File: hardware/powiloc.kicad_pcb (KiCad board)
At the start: 2 copper layers, 55.9 x 92.7 mm, 46 parts, among them J1 SW_PWR_BAT, J2 MCU_ISP, J3 SW_ISP_MCU, J4 neo_gps_conn, J5 oled_conn, J6 periph_conn_1, J7 BATT, J8 radio_ant_conn**, J9 MCU_TX, Q1 IRF740, Q2 IRF740, SW1 SW_TRIG, SW2 SW_MAIN_RST, SW3 SW_LED_PWR, SW4 SW_LED_STAT, SW5 SW_RADIO_RST, U1 MCP1700, U2 USB Conn, U3 RFM95W, U4 328p_main, U5 328p_radio, Y1 12MHz

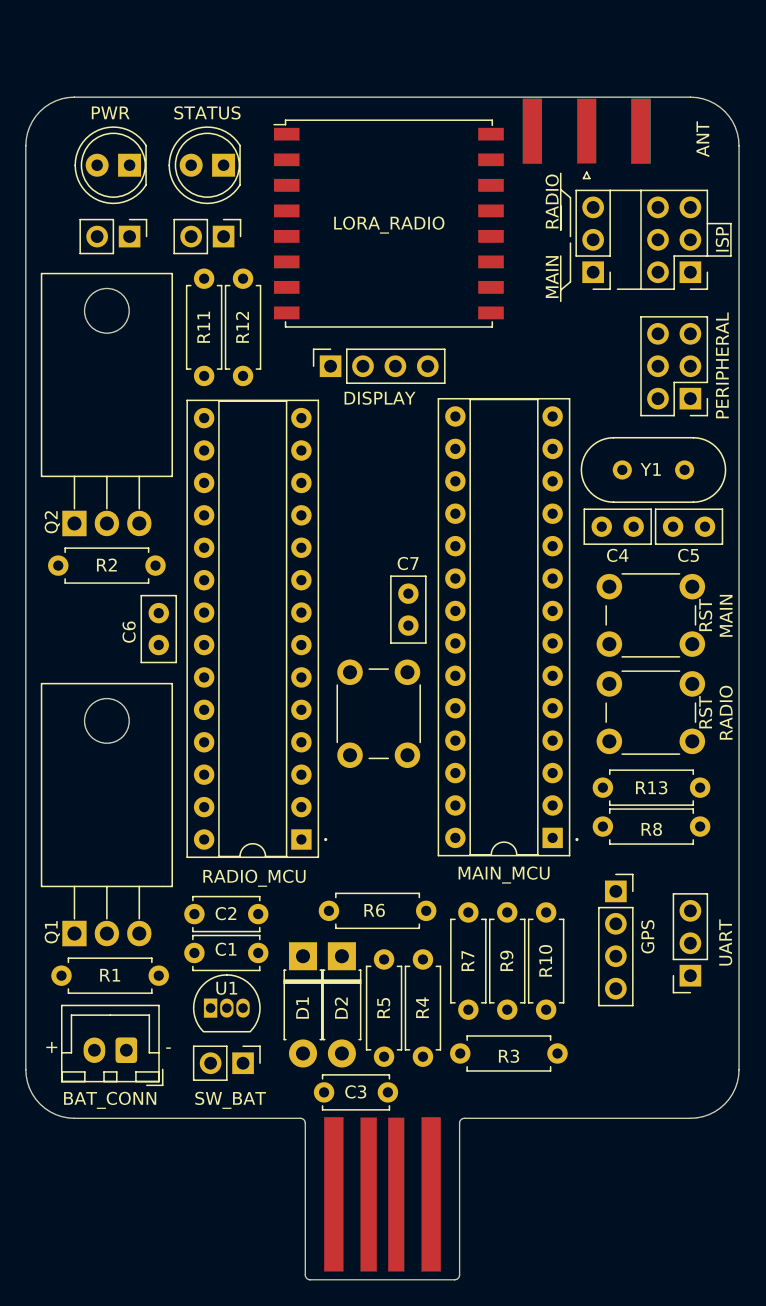
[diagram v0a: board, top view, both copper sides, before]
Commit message: Corrupt save
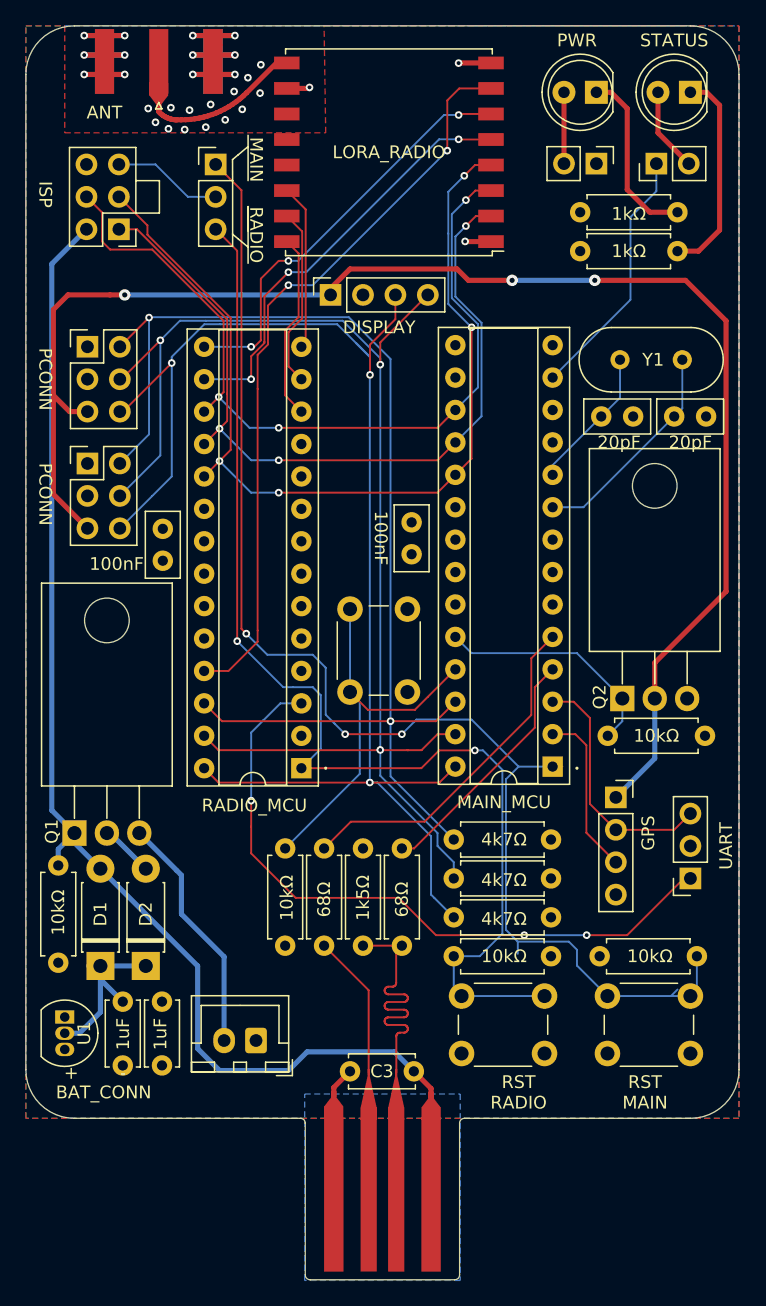
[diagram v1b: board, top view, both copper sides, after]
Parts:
- added T1: taper, powiloc-custom:uwT0.50_0.40_1.00_1.46_1.20, F.Cu at (146.1, 137.9)
- added T2: taper, powiloc-custom:uwT0.50_0.40_1.00_1.46_1.20, F.Cu at (138.4, 137.8)
- added T3: taper, powiloc-custom:uwT0.50_0.15_1.00_1.24_3.00, F.Cu at (141.2, 136.1)
- added T4: taper, powiloc-custom:uwT0.50_0.15_1.00_1.24_3.00, F.Cu at (143.3, 136.1)
- added T5: taper, powiloc-custom:uwT0.50_0.40_1.00_1.46_1.20, F.Cu at (124.7, 60.5)
- J1: value SW_PWR_BAT -> periph_conn_2; footprint Connector_PinHeader_2.54mm:PinHeader_1x02_P2.54mm_Vertical -> Connector_PinHeader_2.54mm:PinHeader_2x03_P2.54mm_Vertical
- moved J1 48.5 mm to (119.1, 88.4), turned to 0 degrees
- moved J6 47.4 mm to (119.1, 79.2), turned to 0 degrees
- moved R2 45.1 mm to (167.5, 109.7)
- moved Q2 45.1 mm to (161.0, 106.8)
- moved J2 44.9 mm to (121.6, 70.0)
- moved SW2 37.1 mm to (166.4, 134.6), turned to 180 degrees
- moved D3 37.0 mm to (159.0, 59.3)
- moved D4 37.0 mm to (166.4, 59.3)
- moved SW3 37.0 mm to (159.0, 64.9)
- moved SW4 34.4 mm to (163.7, 64.9), turned to 90 degrees
- moved J8 34.0 mm to (124.7, 56.9)
- moved R11 32.1 mm to (157.7, 68.7), turned to 0 degrees
- moved J3 30.8 mm to (129.2, 65.0), turned to 0 degrees
- moved SW5 29.4 mm to (154.9, 134.6), turned to 180 degrees
- moved R12 28.2 mm to (157.7, 71.8), turned to 0 degrees
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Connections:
- J1 pad 1: BAT+ -> 3.3V
- J1 pad 2: Net-(J1-Pad2) -> I2C_SMBALERT
- Q1 pad 3: Net-(J1-Pad2) -> BAT+
- U4 pad 4: USB_D+ -> USB_D-
- U4 pad 5: USB_D- -> USB_D+
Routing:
- net 3.3V_SW: track 0.00 -> 118.4 mm, vias 0 -> 3
- net I2C_SCL: track 0.00 -> 114.7 mm, vias 0 -> 3
- net I2C_SDA: track 0.00 -> 109.2 mm, vias 0 -> 3
- net NRST_MAIN_MCU: track 0.00 -> 104.8 mm, vias 0 -> 3
- net VBUS: track 0.00 -> 102.2 mm
- net I2C_SMBALERT: track 0.00 -> 97.1 mm, vias 0 -> 2
- net NRST_RADIO_MCU: track 0.00 -> 91.8 mm, vias 0 -> 2
- net BAT-: track 0.00 -> 87.0 mm, vias 0 -> 29
- net SPI_SCK: track 0.00 -> 74.2 mm, vias 0 -> 4
- net SPI_MOSI: track 0.00 -> 64.7 mm, vias 0 -> 3
- net SPI_MISO: track 0.00 -> 63.3 mm, vias 0 -> 3
- net RADIO_DIO5: track 0.00 -> 58.6 mm, vias 0 -> 2
- net RADIO_TX: track 0.00 -> 53.3 mm, vias 0 -> 3
- net RADIO_NSS: track 0.00 -> 33.5 mm, vias 0 -> 3
- net RADIO_RST: track 0.00 -> 32.9 mm, vias 0 -> 3
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- added copper zone on F.Cu, net 3.3V
- added copper zone on B.Cu, net BAT-
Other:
- board size 55.9 x 92.7 mm -> 55.9 x 98.2 mm
- board text added: "+sw"
- board text added: "100nF"
- board text added: "10kΩ"
- board text added: "1k5Ω"
- board text added: "1kΩ"
- board text added: "1uF"
- board text added: "20pF"
- board text added: "4k7Ω"
- board text added: "68Ω"
- board text added: "ALERT"
- board text added: "MAIN_TX"
- board text added: "PCONN"
- board text added: "RADIO_TX"
- board text removed: "++"
- board text removed: "PERIPHERAL"
- board text removed: "SMBALERT"
- board text removed: "SW_BAT"
